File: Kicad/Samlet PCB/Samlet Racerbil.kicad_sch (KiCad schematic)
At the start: 11 parts, among them J1 Pickit Forbindelse, J5 Conn_01x05_Female, Q1 IRL1404, U2 PIC16F684-IP

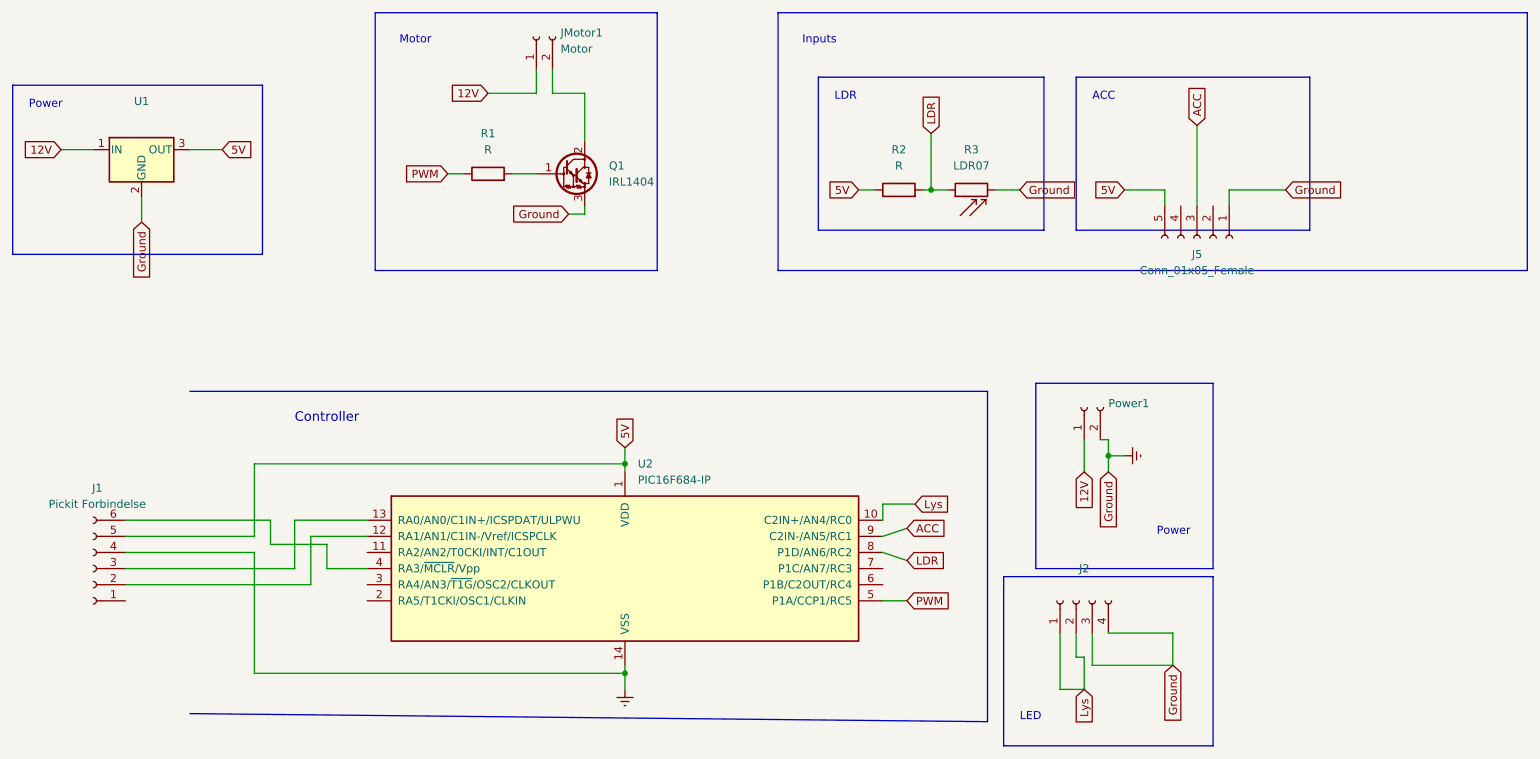
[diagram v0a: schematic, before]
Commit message: Capacitor
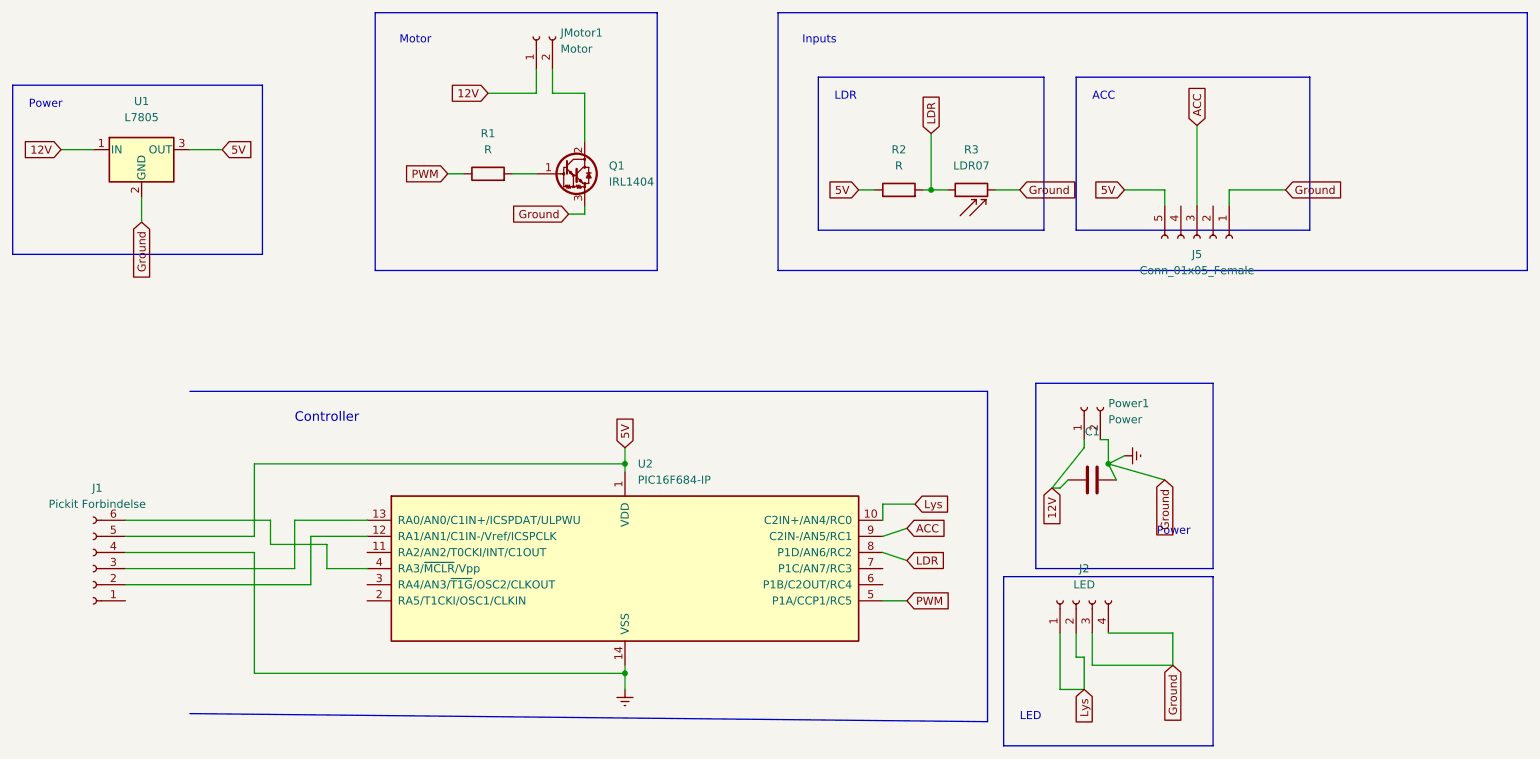
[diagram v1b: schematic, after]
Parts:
- added C1: (no value), symbol Device:C
- J2: value (none) -> LED; footprint (none) -> Connector_PinHeader_2.54mm:PinHeader_1x04_P2.54mm_Vertical
- Power1: value (none) -> Power
- U1: value (none) -> L7805; footprint (none) -> Package_TO_SOT_THT:TO-220-3_Vertical
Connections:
- net 12V: now also C1.1
- net Earth: now also C1.2
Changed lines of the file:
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@@
 (kicad_sch (version 20211123) (generator eeschema)
   (paper "A4")
-  (junction (at 212.09 92.71) (diameter 0) (color 0 0 0 0)
+  (junction (at 212.09 93.98) (diameter 0) (color 0 0 0 0)
   )
   (junction (at 184.15 50.8) (diameter 0) (color 0 0 0 0)
@@
     (stroke (width 0) (type default) (color 0 0 0 0))
   )
-  (wire (pts (xy 208.28 90.17) (xy 208.28 95.25))
+  (wire (pts (xy 208.28 91.44) (xy 203.2 97.79))
     (stroke (width 0) (type default) (color 0 0 0 0))
   )
@@
     (stroke (width 0) (type default) (color 0 0 0 0))
   )
+  (wire (pts (xy 204.47 97.79) (xy 203.2 97.79))
+    (stroke (width 0) (type default) (color 0 0 0 0))
+  )
   (wire (pts (xy 220.98 50.8) (xy 220.98 53.34))
     (stroke (width 0) (type default) (color 0 0 0 0))
   )
-  (wire (pts (xy 212.09 92.71) (xy 212.09 90.17))
+  (wire (pts (xy 212.09 93.98) (xy 212.09 90.17))
     (stroke (width 0) (type default) (color 0 0 0 0))
   )
@@
     (stroke (width 0) (type default) (color 0 0 0 0))
   )
+  (wire (pts (xy 208.28 91.44) (xy 208.28 90.17))
+    (stroke (width 0) (type default) (color 0 0 0 0))
+  )
   (wire (pts (xy 118.11 48.26) (xy 121.92 48.26))
     (stroke (width 0) (type default) (color 0 0 0 0))
@@
     (stroke (width 0) (type default) (color 0 0 0 0))
   )
-  (wire (pts (xy 212.09 95.25) (xy 212.09 92.71))
+  (wire (pts (xy 220.98 96.52) (xy 212.09 93.98))
     (stroke (width 0) (type default) (color 0 0 0 0))
   )
@@
     (stroke (width 0) (type default) (color 0 0 0 0))
   )
-  (wire (pts (xy 212.09 92.71) (xy 214.63 92.71))
+  (wire (pts (xy 212.09 93.98) (xy 214.63 92.71))
+    (stroke (width 0) (type default) (color 0 0 0 0))
+  )
+  (wire (pts (xy 205.74 96.52) (xy 204.47 97.79))
     (stroke (width 0) (type default) (color 0 0 0 0))
   )
@@
   )
   (polyline (pts (xy 207.01 33.02) (xy 243.84 33.02))
+    (stroke (width 0) (type default) (color 0 0 0 0))
+  )
+  (wire (pts (xy 213.36 96.52) (xy 212.09 93.98))
     (stroke (width 0) (type default) (color 0 0 0 0))
   )
@@
     )
   )
-  (global_label "Ground" (shape input) (at 212.09 95.25 270) (fields_autoplaced)
-    (effects (font (size 1.27 1.27)) (justify right))
-    (property "Intersheet References" "${INTERSHEET_REFS}" (id 0) (at 212.1694 104.3155 90)
+  (global_label "Ground" (shape input) (at 220.98 96.52 270) (fields_autoplaced)
+    (effects (font (size 1.27 1.27)) (justify right))
+    (property "Intersheet References" "${INTERSHEET_REFS}" (id 0) (at 221.0594 105.5855 90)
       (effects (font (size 1.27 1.27)) (justify right) hide)
     )
@@
     )
   )
-  (global_label "12V" (shape input) (at 208.28 95.25 270) (fields_autoplaced)
-    (effects (font (size 1.27 1.27)) (justify right))
-    (property "Intersheet References" "${INTERSHEET_REFS}" (id 0) (at 208.2006 101.1707 90)
+  (global_label "12V" (shape input) (at 203.2 97.79 270) (fields_autoplaced)
+    (effects (font (size 1.27 1.27)) (justify right))
+    (property "Intersheet References" "${INTERSHEET_REFS}" (id 0) (at 203.1206 103.7107 90)
       (effects (font (size 1.27 1.27)) (justify right) hide)
     )
@@
     (pin "1")
   )
+  (symbol (lib_id "Device:C") (at 209.55 96.52 90) (unit 1)
+    (in_bom yes) (on_board yes) (fields_autoplaced)
+    (property "Reference" "C1" (id 0) (at 209.55 88.9 90))
+    (property "Value" "" (id 1) (at 209.55 91.44 90))
+    (property "Footprint" "" (id 2) (at 213.36 95.5548 0)
+      (effects (font (size 1.27 1.27)) hide)
+    )
+    (property "Datasheet" "~" (id 3) (at 209.55 96.52 0)
+      (effects (font (size 1.27 1.27)) hide)
+    )
+    (pin "1")
+    (pin "2")
+  )
   (symbol (lib_id "Connector:Conn_01x02_Female") (at 208.28 85.09 90) (unit 1)
     (in_bom yes) (on_board yes) (fields_autoplaced)
@@
       (effects (font (size 1.27 1.27)) (justify right))
     )
-    (property "Value" "" (id 1) (at 212.09 86.9949 90)
+    (property "Value" "Power" (id 1) (at 212.09 86.9949 90)
       (effects (font (size 1.27 1.27)) (justify right))
     )
@@
     (in_bom yes) (on_board yes) (fields_autoplaced)
     (property "Reference" "U1" (id 0) (at 59.69 36.83 0))
-    (property "Value" "" (id 1) (at 59.69 39.37 0))
-    (property "Footprint" "" (id 2) (at 60.325 48.26 0)
+    (property "Value" "L7805" (id 1) (at 59.69 39.37 0))
+    (property "Footprint" "Package_TO_SOT_THT:TO-220-3_Vertical" (id 2) (at 60.325 48.26 0)
       (effects (font (size 1.27 1.27) italic) (justify left) hide)
     )
@@
     (in_bom yes) (on_board yes) (fields_autoplaced)
     (property "Reference" "J2" (id 0) (at 208.28 110.49 90))
-    (property "Value" "" (id 1) (at 208.28 113.03 90))
-    (property "Footprint" "" (id 2) (at 207.01 115.57 0)
+    (property "Value" "LED" (id 1) (at 208.28 113.03 90))
+    (property "Footprint" "Connector_PinHeader_2.54mm:PinHeader_1x04_P2.54mm_Vertical" (id 2) (at 207.01 115.57 0)
       (effects (font (size 1.27 1.27)) hide)
     )
@@
       (reference "#PWR0103") (unit 1) (value "Earth") (footprint "")
     )
+    (path "/bd72fe48-0065-44ec-a7be-6c365f617f93"
+      (reference "C1") (unit 1) (value "C") (footprint "Capacitor_THT:CP_Radial_D7.5mm_P2.50mm")
+    )
     (path "/087273d8-55b6-4020-845a-2d45bb9eeebd"

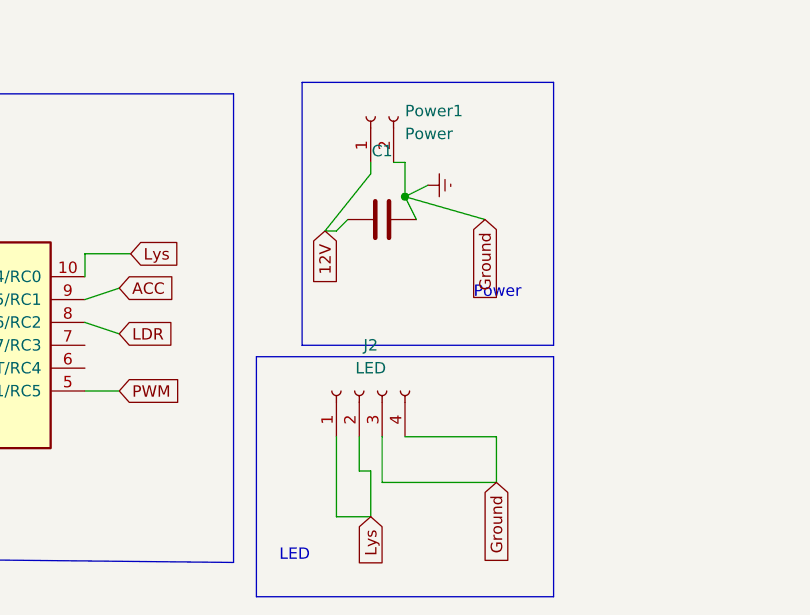
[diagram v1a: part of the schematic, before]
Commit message: h
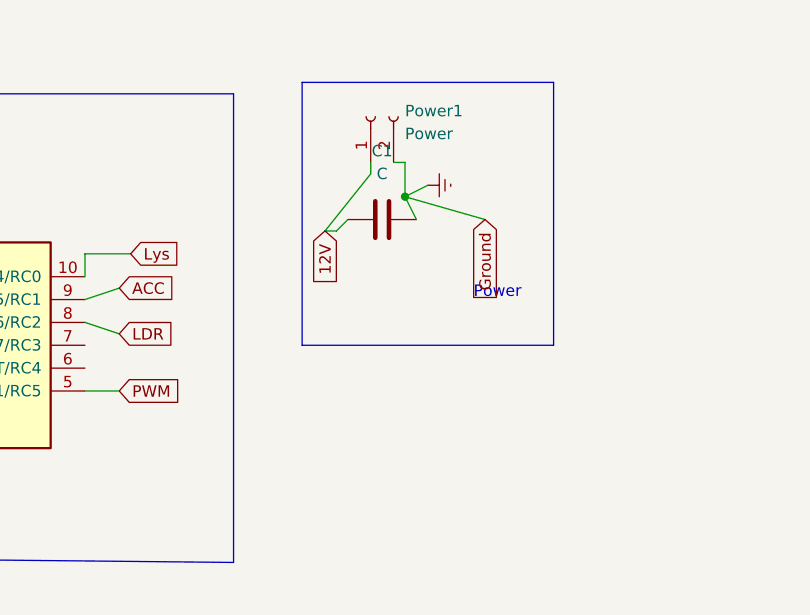
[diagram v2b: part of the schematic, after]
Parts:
- removed J2: LED, Connector_PinHeader_2.54mm:PinHeader_1x04_P2.54mm_Vertical, symbol Connector:Conn_01x04_Female
- C1: value (none) -> C; footprint (none) -> Capacitor_THT:CP_Radial_D7.5mm_P2.50mm
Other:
- note removed: "LED"
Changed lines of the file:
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@@
-    (stroke (width 0) (type default) (color 0 0 0 0))
-  )
-  (wire (pts (xy 209.55 120.65) (xy 209.55 125.73))
     (stroke (width 0) (type default) (color 0 0 0 0))
   )
@@
     (stroke (width 0) (type default) (color 0 0 0 0))
   )
-  (wire (pts (xy 208.28 129.54) (xy 208.28 124.46))
-    (stroke (width 0) (type default) (color 0 0 0 0))
-  )
   (wire (pts (xy 214.63 50.8) (xy 220.98 50.8))
     (stroke (width 0) (type default) (color 0 0 0 0))
@@
     (stroke (width 0) (type default) (color 0 0 0 0))
   )
-  (wire (pts (xy 204.47 129.54) (xy 204.47 120.65))
-    (stroke (width 0) (type default) (color 0 0 0 0))
-  )
   (wire (pts (xy 172.72 50.8) (xy 175.26 50.8))
     (stroke (width 0) (type default) (color 0 0 0 0))
@@
     (stroke (width 0) (type default) (color 0 0 0 0))
   )
-  (wire (pts (xy 208.28 124.46) (xy 207.01 124.46))
-    (stroke (width 0) (type default) (color 0 0 0 0))
-  )
   (polyline (pts (xy 39.37 34.29) (xy 78.74 34.29))
     (stroke (width 0) (type default) (color 0 0 0 0))
@@
     (stroke (width 0) (type default) (color 0 0 0 0))
   )
-  (wire (pts (xy 208.28 129.54) (xy 204.47 129.54))
-    (stroke (width 0) (type default) (color 0 0 0 0))
-  )
   (wire (pts (xy 88.9 110.49) (xy 88.9 106.68))
     (stroke (width 0) (type default) (color 0 0 0 0))
@@
     (stroke (width 0) (type default) (color 0 0 0 0))
   )
-  (polyline (pts (xy 228.6 138.43) (xy 195.58 138.43))
-    (stroke (width 0) (type default) (color 0 0 0 0))
-  )
   (wire (pts (xy 176.53 102.87) (xy 176.53 100.33))
     (stroke (width 0) (type default) (color 0 0 0 0))
@@
     (stroke (width 0) (type default) (color 0 0 0 0))
   )
-  (wire (pts (xy 207.01 124.46) (xy 207.01 120.65))
-    (stroke (width 0) (type default) (color 0 0 0 0))
-  )
   (wire (pts (xy 80.01 106.68) (xy 80.01 102.87))
     (stroke (width 0) (type default) (color 0 0 0 0))
@@
     (stroke (width 0) (type default) (color 0 0 0 0))
   )
-  (wire (pts (xy 212.09 120.65) (xy 222.25 120.65))
-    (stroke (width 0) (type default) (color 0 0 0 0))
-  )
   (wire (pts (xy 176.53 100.33) (xy 181.61 100.33))
     (stroke (width 0) (type default) (color 0 0 0 0))
@@
     (stroke (width 0) (type default) (color 0 0 0 0))
   )
-  (polyline (pts (xy 195.58 111.76) (xy 195.58 138.43))
-    (stroke (width 0) (type default) (color 0 0 0 0))
-  )
   (wire (pts (xy 57.15 102.87) (xy 80.01 102.87))
     (stroke (width 0) (type default) (color 0 0 0 0))
@@
     (stroke (width 0) (type default) (color 0 0 0 0))
   )
-  (polyline (pts (xy 228.6 111.76) (xy 228.6 138.43))
-    (stroke (width 0) (type default) (color 0 0 0 0))
-  )
   (wire (pts (xy 121.92 35.56) (xy 121.92 31.75))
     (stroke (width 0) (type default) (color 0 0 0 0))
@@
   )
   (wire (pts (xy 176.53 105.41) (xy 180.34 104.14))
-    (stroke (width 0) (type default) (color 0 0 0 0))
-  )
-  (wire (pts (xy 209.55 125.73) (xy 222.25 125.73))
-    (stroke (width 0) (type default) (color 0 0 0 0))
-  )
-  (polyline (pts (xy 195.58 111.76) (xy 228.6 111.76))
-    (stroke (width 0) (type default) (color 0 0 0 0))
-  )
-  (wire (pts (xy 222.25 120.65) (xy 222.25 125.73))
     (stroke (width 0) (type default) (color 0 0 0 0))
   )
@@
     (effects (font (size 1.27 1.27)) (justify left bottom))
   )
-  (text "LED\n" (at 198.12 134.62 0)
-    (effects (font (size 1.27 1.27)) (justify left bottom))
-  )
   (text "Motor\n" (at 100.33 27.94 0)
     (effects (font (size 1.27 1.27)) (justify left bottom))
@@
     )
   )
-  (global_label "Ground" (shape input) (at 222.25 125.73 270) (fields_autoplaced)
-    (effects (font (size 1.27 1.27)) (justify right))
-    (property "Intersheet References" "${INTERSHEET_REFS}" (id 0) (at 222.3294 134.7955 90)
-      (effects (font (size 1.27 1.27)) (justify right) hide)
-    )
-  )
   (global_label "ACC" (shape input) (at 226.06 40.64 90) (fields_autoplaced)
     (effects (font (size 1.27 1.27)) (justify left))
@@
     (effects (font (size 1.27 1.27)) (justify right))
     (property "Intersheet References" "${INTERSHEET_REFS}" (id 0) (at 41.0693 44.3706 0)
-      (effects (font (size 1.27 1.27)) (justify right) hide)
-    )
-  )
-  (global_label "Lys" (shape input) (at 208.28 129.54 270) (fields_autoplaced)
-    (effects (font (size 1.27 1.27)) (justify right))
-    (property "Intersheet References" "${INTERSHEET_REFS}" (id 0) (at 208.3594 134.9769 90)
       (effects (font (size 1.27 1.27)) (justify right) hide)
     )
@@
     (in_bom yes) (on_board yes) (fields_autoplaced)
     (property "Reference" "C1" (id 0) (at 209.55 88.9 90))
-    (property "Value" "" (id 1) (at 209.55 91.44 90))
-    (property "Footprint" "" (id 2) (at 213.36 95.5548 0)
+    (property "Value" "C" (id 1) (at 209.55 91.44 90))
+    (property "Footprint" "Capacitor_THT:CP_Radial_D7.5mm_P2.50mm" (id 2) (at 213.36 95.5548 0)
       (effects (font (size 1.27 1.27)) hide)
     )
@@
     (pin "2")
   )
-  (symbol (lib_id "Connector:Conn_01x04_Female") (at 207.01 115.57 90) (unit 1)
-    (in_bom yes) (on_board yes) (fields_autoplaced)
-    (property "Reference" "J2" (id 0) (at 208.28 110.49 90))
-    (property "Value" "LED" (id 1) (at 208.28 113.03 90))
-    (property "Footprint" "Connector_PinHeader_2.54mm:PinHeader_1x04_P2.54mm_Vertical" (id 2) (at 207.01 115.57 0)
-      (effects (font (size 1.27 1.27)) hide)
-    )
-    (property "Datasheet" "~" (id 3) (at 207.01 115.57 0)
-      (effects (font (size 1.27 1.27)) hide)
-    )
-    (pin "1")
-    (pin "2")
-    (pin "3")
-    (pin "4")
-  )
   (sheet_instances
     (path "/" (page "1"))
@@
       (reference "J1") (unit 1) (value "Pickit Forbindelse") (footprint "Connector_PinHeader_2.54mm:PinHeader_1x06_P2.54mm_Vertical")
     )
-    (path "/f1941a35-e4e9-42e3-af20-b900f5caf889"
-      (reference "J2") (unit 1) (value "LED") (footprint "Connector_PinHeader_2.54mm:PinHeader_1x04_P2.54mm_Vertical")
-    )
     (path "/7800d3be-c041-4b10-8108-1cf92520b594"
